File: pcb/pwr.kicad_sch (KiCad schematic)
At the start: 34 parts, among them J2 Adafruit Wireless Chg Module, SW6 PWR, U4 TPS63802DLAR, U5 TPS7A20xxxDQN, U6 BQ24074RGT, U7 MCP73831-2-OT, U9 TPS2116DRL

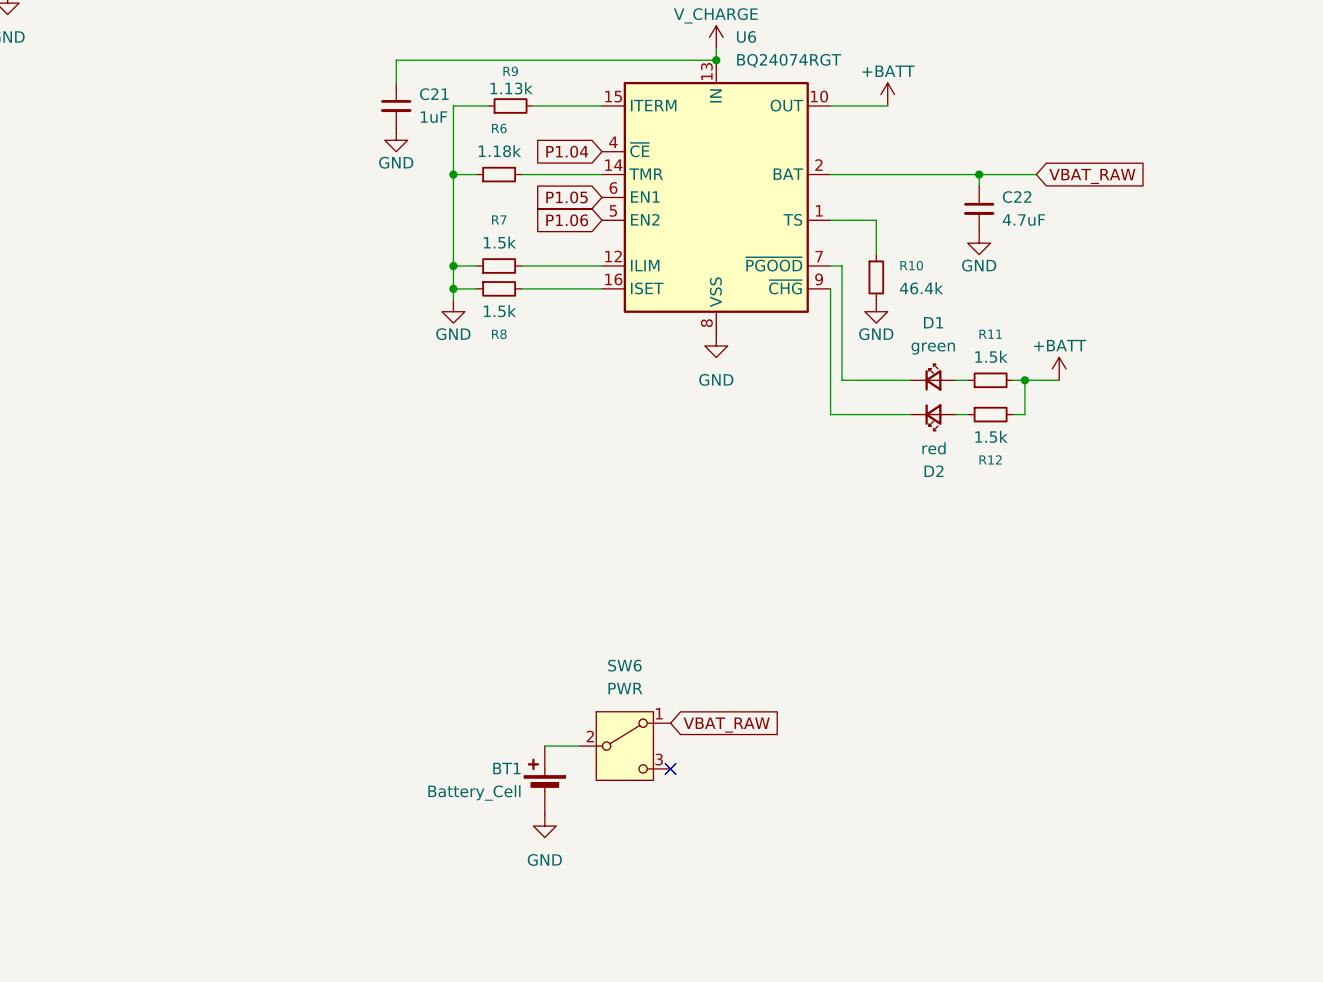
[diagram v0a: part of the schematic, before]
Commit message: starting le leyout
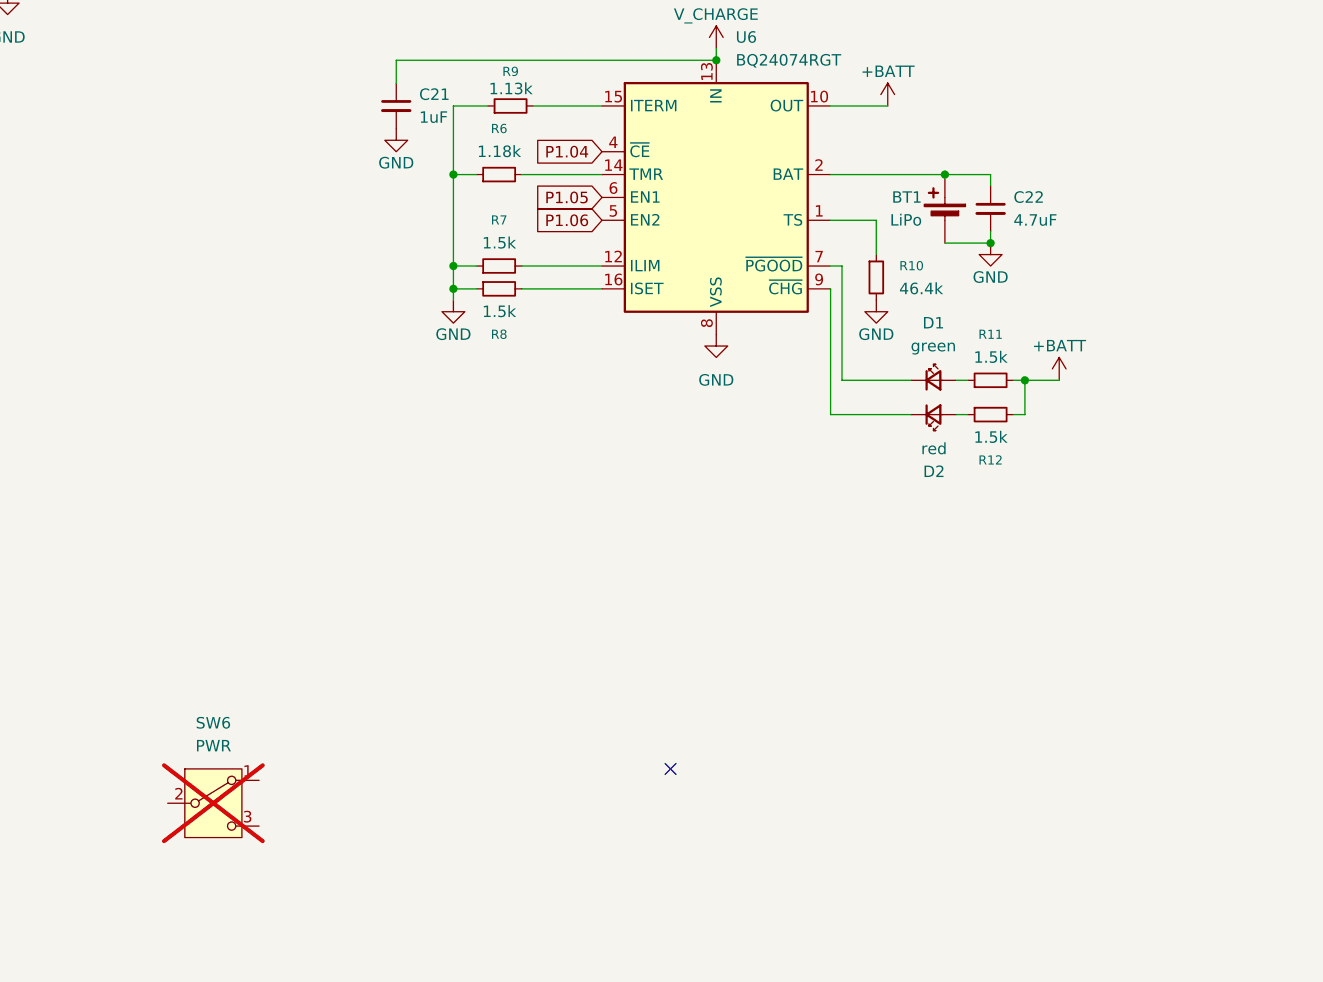
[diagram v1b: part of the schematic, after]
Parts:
- BT1: value Battery_Cell -> LiPo
- SW6: now not fitted; now left out of the parts list
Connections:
- net at BT1.1 (+): now also C22.1, U6.2 (BAT), U6.3 (BAT); no longer SW6.2 (B)
- removed net VBAT_RAW: C22.1, SW6.1 (A), U6.2 (BAT), U6.3 (BAT)
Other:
- moved on the sheet: C22
